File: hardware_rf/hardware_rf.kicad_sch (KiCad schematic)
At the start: 60 parts, among them IC1 CC1125RHBR, IC2 BALF-SPI2-02D3, IC3 4259-63, J1 Conn_Coaxial, J2 Conn_01x03_Socket, SW1 SW_Push, U1 RP2350A-QFN60, U2 W25Q128JVS, Y1 Crystal_GND24, Y2 Crystal_GND24

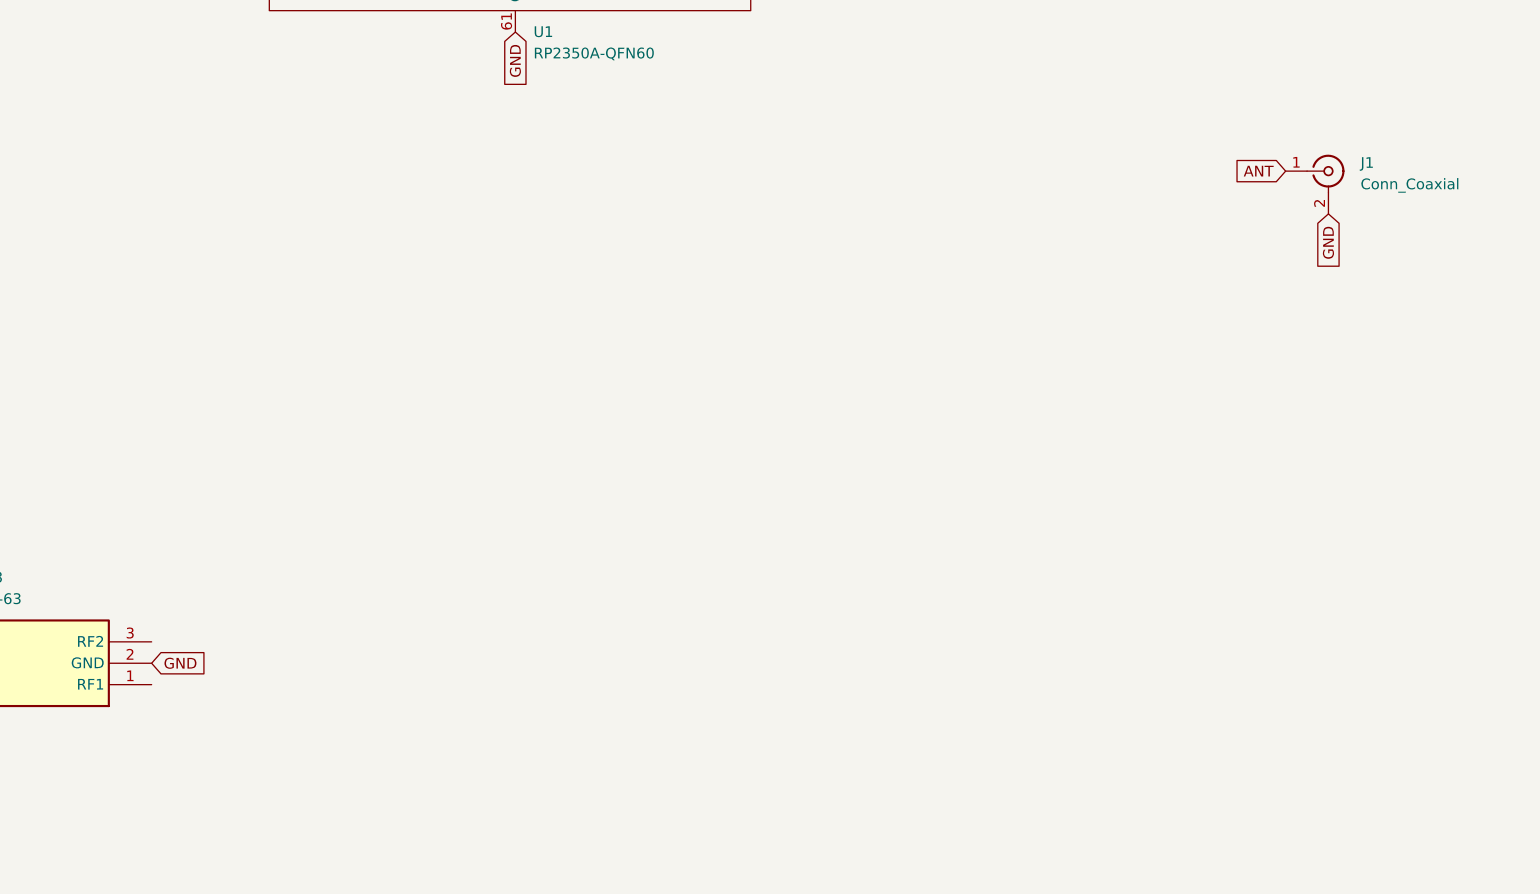
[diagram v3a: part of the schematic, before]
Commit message: sch
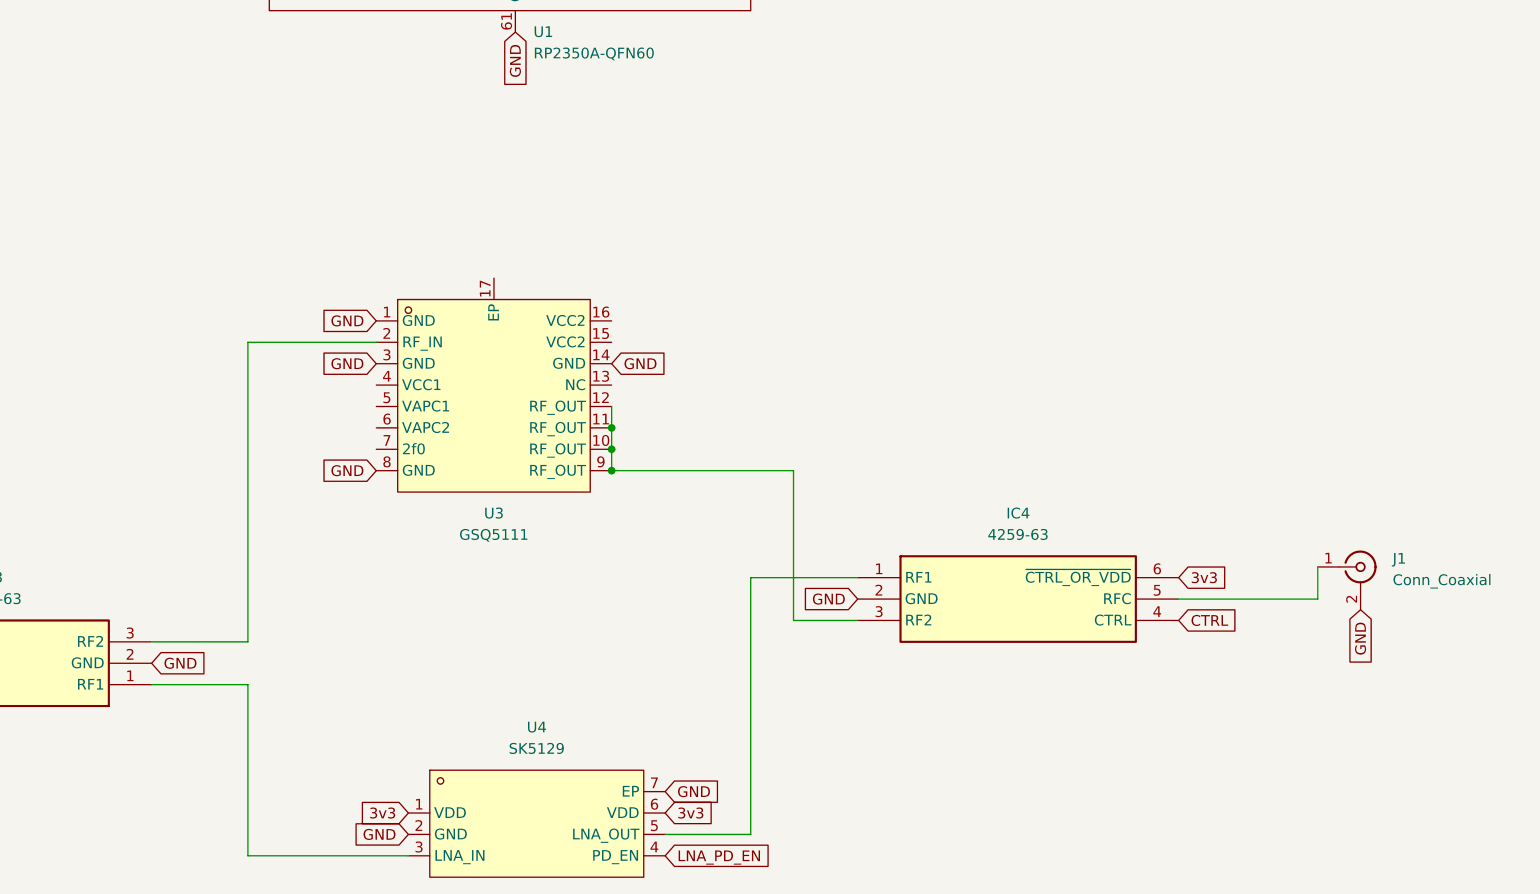
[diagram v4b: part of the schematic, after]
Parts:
- added IC4: 4259-63, mainfoot:PE4259, symbol mainlib:4259-63
- added U3: GSQ5111, easyeda2kicad:QFN-16_L3.0-W3.0-P0.50-TL-EP1.65, symbol easyeda2kicad:GSQ5111
- added U4: SK5129, easyeda2kicad:DFN-6_L1.6-W1.6-P0.50-BL-EP1.0, symbol easyeda2kicad:SK5129
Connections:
- net 3v3: now also IC4.6 (~{CTRL_OR_VDD}), U4.1 (VDD), U4.6 (VDD)
- net CTRL: now also IC4.4 (CTRL)
- net GND: now also IC4.2 (GND), U3.1 (GND), U3.14 (GND), U3.3 (GND), U3.8 (GND), U4.2 (GND), U4.7 (EP)
- net at IC3.1 (RF1): now also U4.3 (LNA_IN)
- net at IC3.3 (RF2): now also U3.2 (RF_IN)
- net ANT: no longer names the net of J1.1 (In)
- net ANT: now also IC4.5 (RFC)
- new net: IC4.3 (RF2), U3.10 (RF_OUT), U3.11 (RF_OUT), U3.12 (RF_OUT), U3.9 (RF_OUT)
- new net: IC4.1 (RF1), U4.5 (LNA_OUT)
- new net LNA_PD_EN: U4.4 (PD_EN)
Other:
- moved on the sheet: J1
